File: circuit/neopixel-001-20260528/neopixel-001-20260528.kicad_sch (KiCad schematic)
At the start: 48 parts, among them J1 Conn_Sub, SW1 SW_SPST, SW2 SW_SPST, SW3 SW_SPST, SW4 SW_SPST

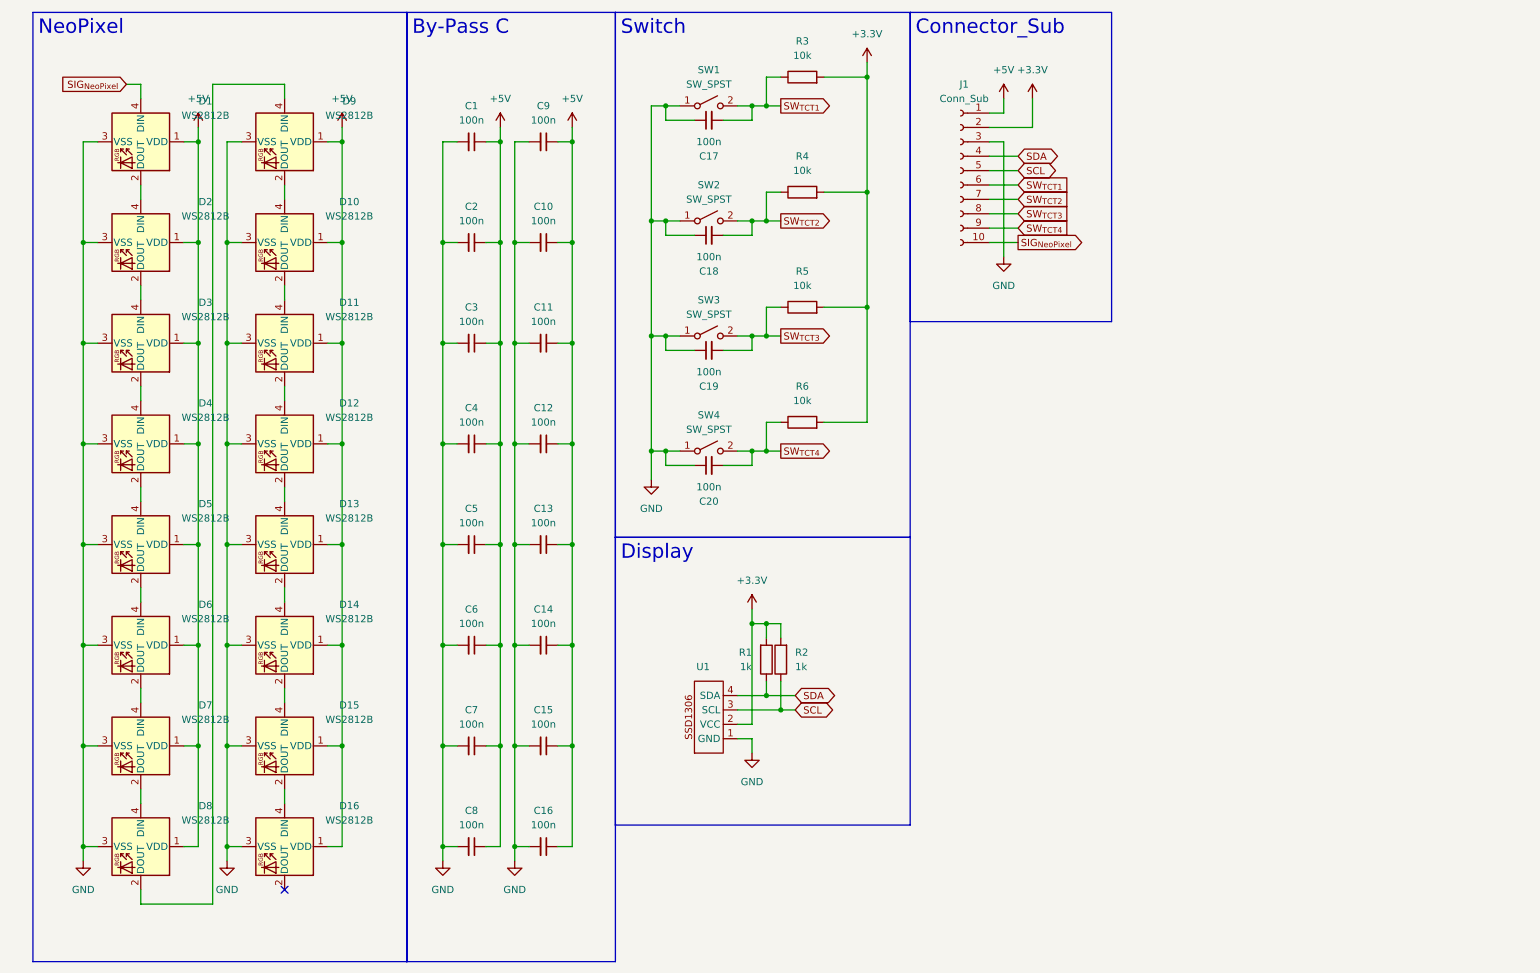
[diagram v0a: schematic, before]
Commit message: Update 供給基板のボード図の修正とDR完了、再DR求
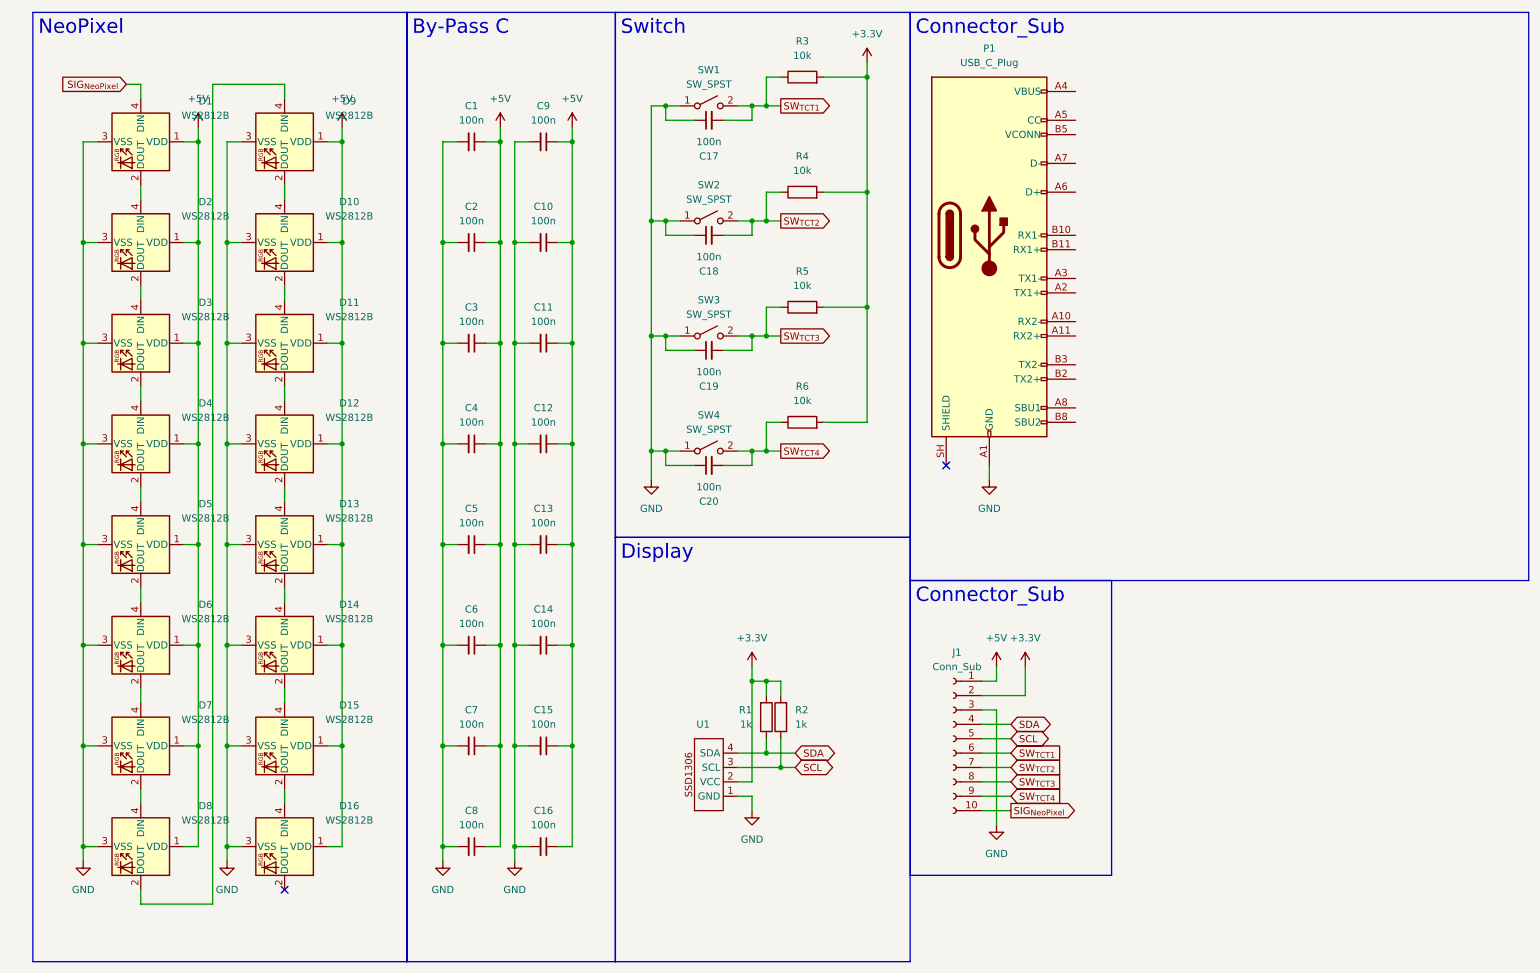
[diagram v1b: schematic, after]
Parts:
- added P1: USB_C_Plug, symbol Connector:USB_C_Plug
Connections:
- net GND: now also P1.A1 (GND), P1.A12 (GND), P1.B1 (GND), P1.B12 (GND)
- new net: P1.A4 (VBUS), P1.A9 (VBUS), P1.B4 (VBUS), P1.B9 (VBUS)
- no-connect marks 1 -> 2
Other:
- moved on the sheet: J1, R1, R2, U1
